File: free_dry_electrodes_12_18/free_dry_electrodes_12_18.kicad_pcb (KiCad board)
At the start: 2 copper layers, 14 x 14 mm, 30 parts

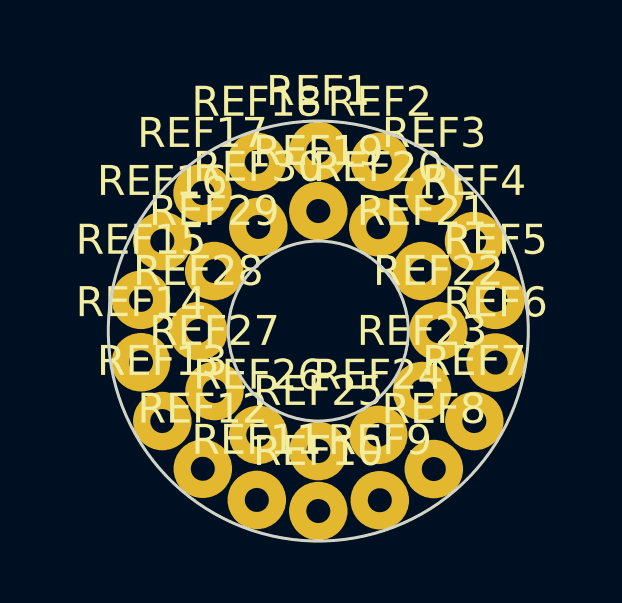
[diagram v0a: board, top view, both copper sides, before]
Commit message: Add files via upload
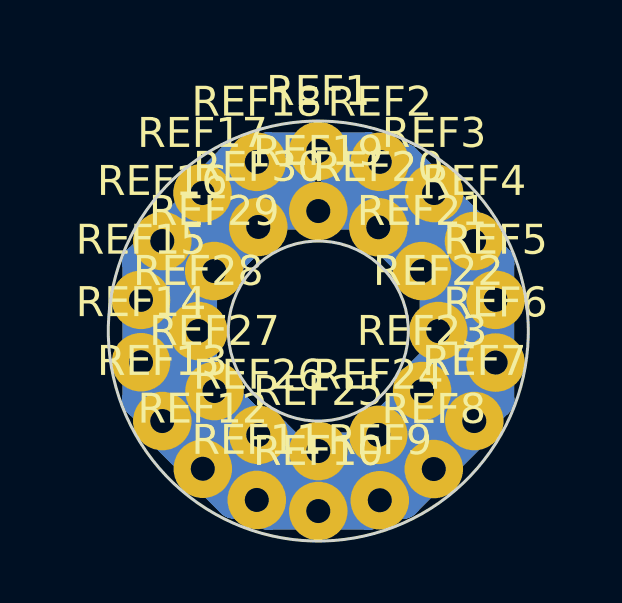
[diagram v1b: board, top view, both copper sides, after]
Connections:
- REF1 pad 1: (no net) -> Net-(REF26-Pad1)
- REF10 pad 1: (no net) -> Net-(REF26-Pad1)
- REF11 pad 1: (no net) -> Net-(REF26-Pad1)
- REF12 pad 1: (no net) -> Net-(REF26-Pad1)
- REF13 pad 1: (no net) -> Net-(REF26-Pad1)
- REF14 pad 1: (no net) -> Net-(REF26-Pad1)
- REF15 pad 1: (no net) -> Net-(REF26-Pad1)
- REF16 pad 1: (no net) -> Net-(REF26-Pad1)
- REF17 pad 1: (no net) -> Net-(REF26-Pad1)
- REF18 pad 1: (no net) -> Net-(REF26-Pad1)
- REF19 pad 1: (no net) -> Net-(REF26-Pad1)
- REF2 pad 1: (no net) -> Net-(REF26-Pad1)
- REF20 pad 1: (no net) -> Net-(REF26-Pad1)
- REF21 pad 1: (no net) -> Net-(REF26-Pad1)
- REF22 pad 1: (no net) -> Net-(REF26-Pad1)
- REF23 pad 1: (no net) -> Net-(REF26-Pad1)
- REF24 pad 1: (no net) -> Net-(REF26-Pad1)
- REF25 pad 1: (no net) -> Net-(REF26-Pad1)
- REF26 pad 1: (no net) -> Net-(REF26-Pad1)
- REF27 pad 1: (no net) -> Net-(REF26-Pad1)
- REF28 pad 1: (no net) -> Net-(REF26-Pad1)
- REF29 pad 1: (no net) -> Net-(REF26-Pad1)
- REF3 pad 1: (no net) -> Net-(REF26-Pad1)
- REF30 pad 1: (no net) -> Net-(REF26-Pad1)
- REF4 pad 1: (no net) -> Net-(REF26-Pad1)
- REF5 pad 1: (no net) -> Net-(REF26-Pad1)
- REF6 pad 1: (no net) -> Net-(REF26-Pad1)
- REF7 pad 1: (no net) -> Net-(REF26-Pad1)
- REF8 pad 1: (no net) -> Net-(REF26-Pad1)
- REF9 pad 1: (no net) -> Net-(REF26-Pad1)
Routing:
- net Net-(REF26-Pad1): track 0.00 -> 203.0 mm
